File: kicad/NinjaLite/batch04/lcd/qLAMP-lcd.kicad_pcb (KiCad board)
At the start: 2 copper layers, 59 x 28.5 mm, 13 parts, among them J1 Conn_01x04_Male, J2 Conn_01x04_Male, J3 Conn_01x04_Male, J4 ALI_Micro_SD_Card, SW1 TACTILE_4, SW2 TACTILE_4, SW3 TACTILE_4

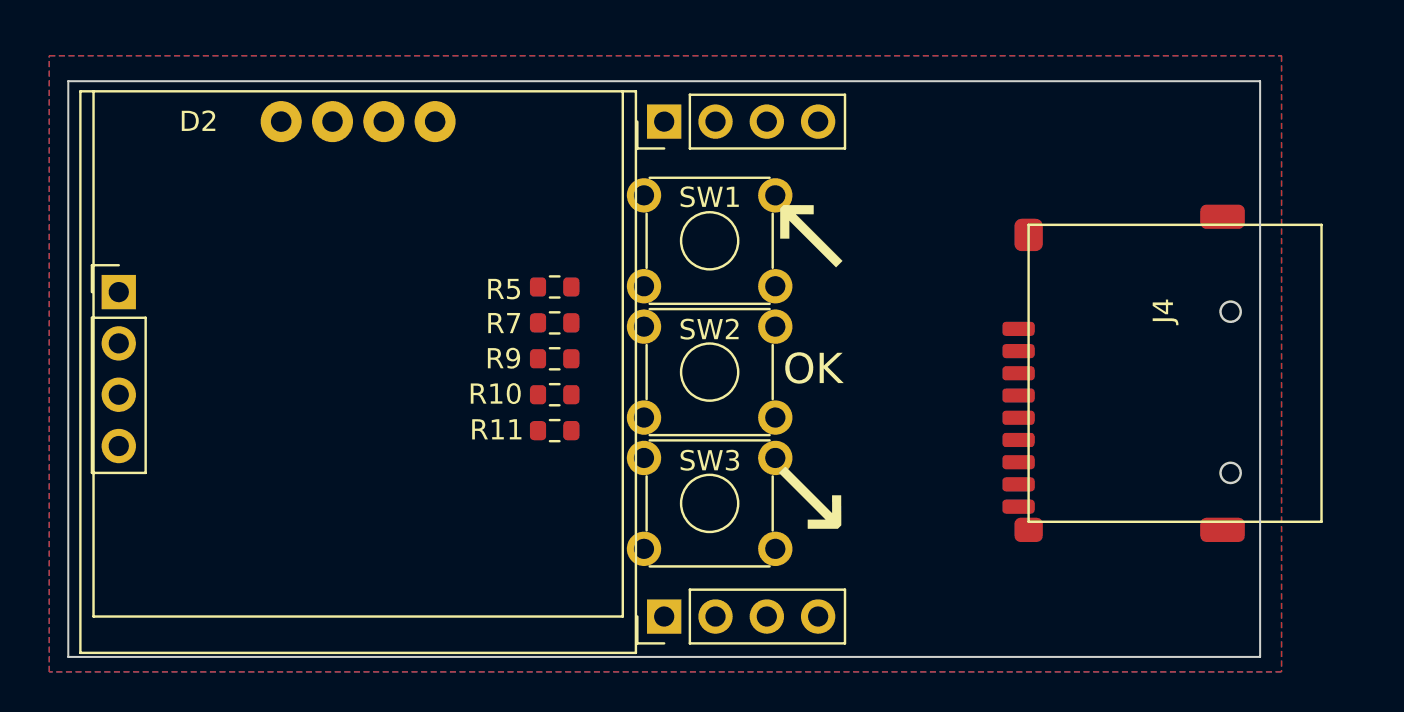
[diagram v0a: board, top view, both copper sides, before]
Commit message: ordered batch04
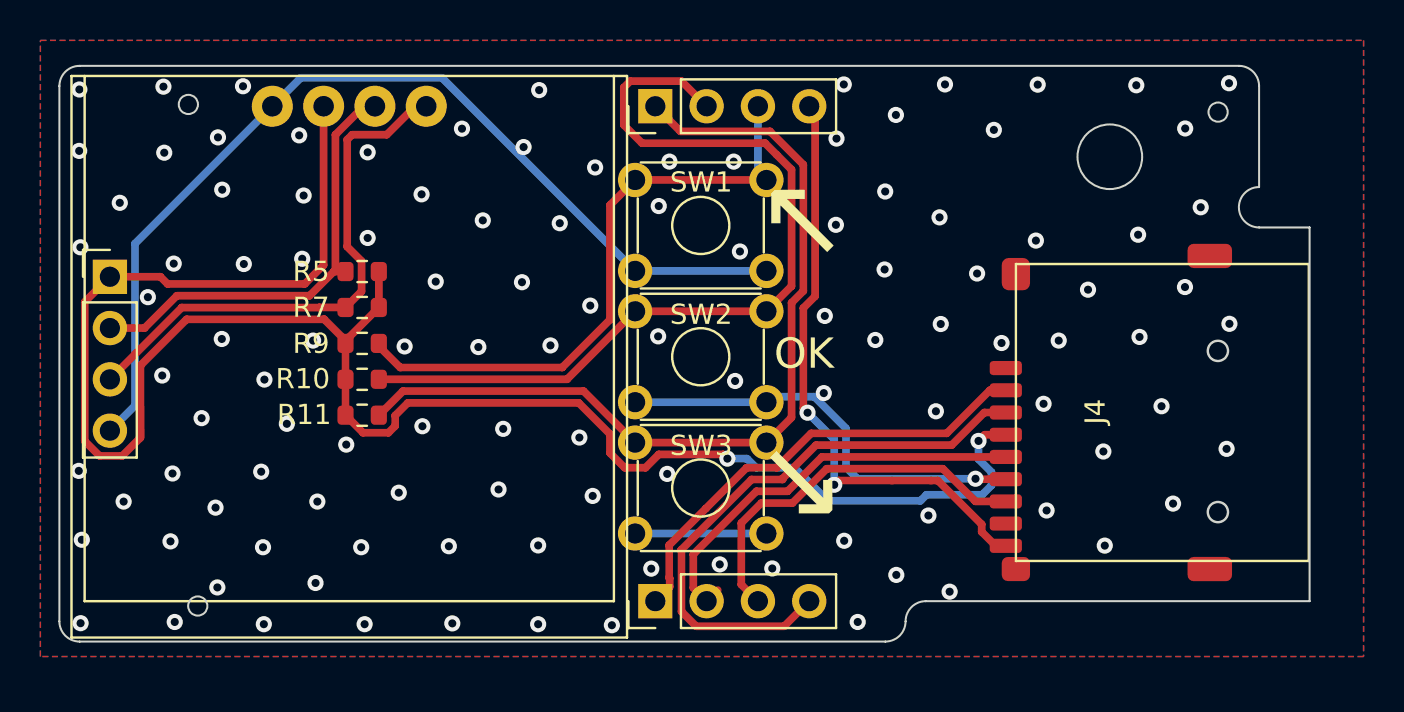
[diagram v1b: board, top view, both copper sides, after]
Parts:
- D2: value ALI_I2C_LCD -> I2C_SSD1306_LCD
- moved R10 9.56 mm to (147.0, 104.0)
- moved R11 9.56 mm to (147.0, 105.8)
- moved R5 9.56 mm to (147.0, 98.7), turned to 180 degrees
- moved R7 9.56 mm to (147.0, 100.5), turned to 180 degrees
- moved R9 9.56 mm to (147.0, 102.2)
- moved J4 2.04 mm to (189.3, 102.6)
- moved J1 0.88 mm to (161.5, 90.5)
- moved J2 0.88 mm to (161.5, 115.0)
- moved J3 0.88 mm to (134.5, 98.9)
- moved D2 0.88 mm to (146.4, 89.0)
- moved SW1 0.88 mm to (160.5, 94.2)
- moved SW2 0.88 mm to (160.5, 100.7)
- moved SW3 0.88 mm to (160.5, 107.2)
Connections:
- net SCL renamed I2C_SCL
- net SDA renamed I2C_SDA
- D2 pad 2: VCC -> 3V3D
- J1 pad 1: SD_CD -> TACT3
- J1 pad 2: SD_CS -> TACT2
- J1 pad 3: MOSI -> TACT1
- J1 pad 4: MISO -> SD_CD
- J2 pad 1: TACT3 -> SD_CS
- J2 pad 2: TACT2 -> SCLK
- J2 pad 3: TACT1 -> MISO
- J2 pad 4: SCLK -> MOSI
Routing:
- net 3V3D: track 0.00 -> 101.8 mm, vias 0 -> 2
- net GND: track 0.00 -> 76.2 mm, vias 0 -> 115
- net TACT2: track 0.00 -> 44.3 mm
- net TACT3: track 0.00 -> 43.8 mm
- net TACT1: track 0.00 -> 30.8 mm
- net SD_CD: track 0.00 -> 29.9 mm, vias 0 -> 2
- net MOSI: track 0.00 -> 29.7 mm
- net I2C_SDA: track 0.00 -> 26.7 mm
- net SD_CS: track 0.00 -> 23.4 mm
- net I2C_SCL: track 0.00 -> 22.3 mm
- net SCLK: track 0.00 -> 20.8 mm
- net MISO: track 0.00 -> 19.1 mm
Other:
- board size 59 x 28.5 mm -> 61.9 x 28.5 mm
- board text added: "61.889x28.5mm"
- board text added: "qNinja Lite batch04/lcd"
- board text removed: "39x28.5mm"
